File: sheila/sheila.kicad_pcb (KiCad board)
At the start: 2 copper layers, 53 parts, among them J1 PT_A, J10 GAIN1_RETURN, J11 OT1_A, J12 OT1_B, J13 SHIELD, J14 U1A_A_1, J15 U1A_K_3, J16 TS_T, J17 TS_B, J18 TS_M, J19 TS_GND, J2 PT_B, J20 U2_K_3, J21 GAIN1_GND, J22 U1A_G_2, J23 U2_S_9, J24 U2_A_7, J3 PT_CT, J4 S2_A, J5 S2_B, J7 U1B_6_A, J8 U1B_8_K, J9 GAIN1_SEND

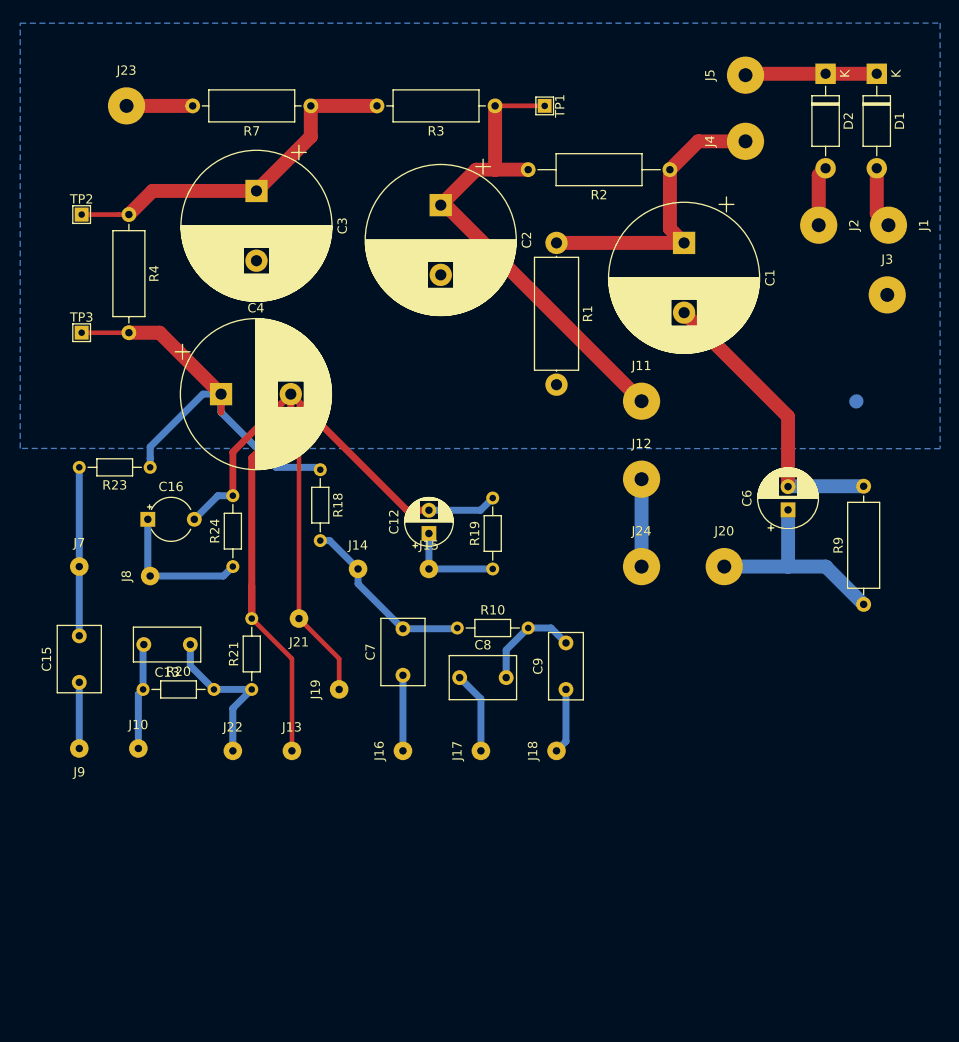
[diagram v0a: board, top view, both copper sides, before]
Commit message: .
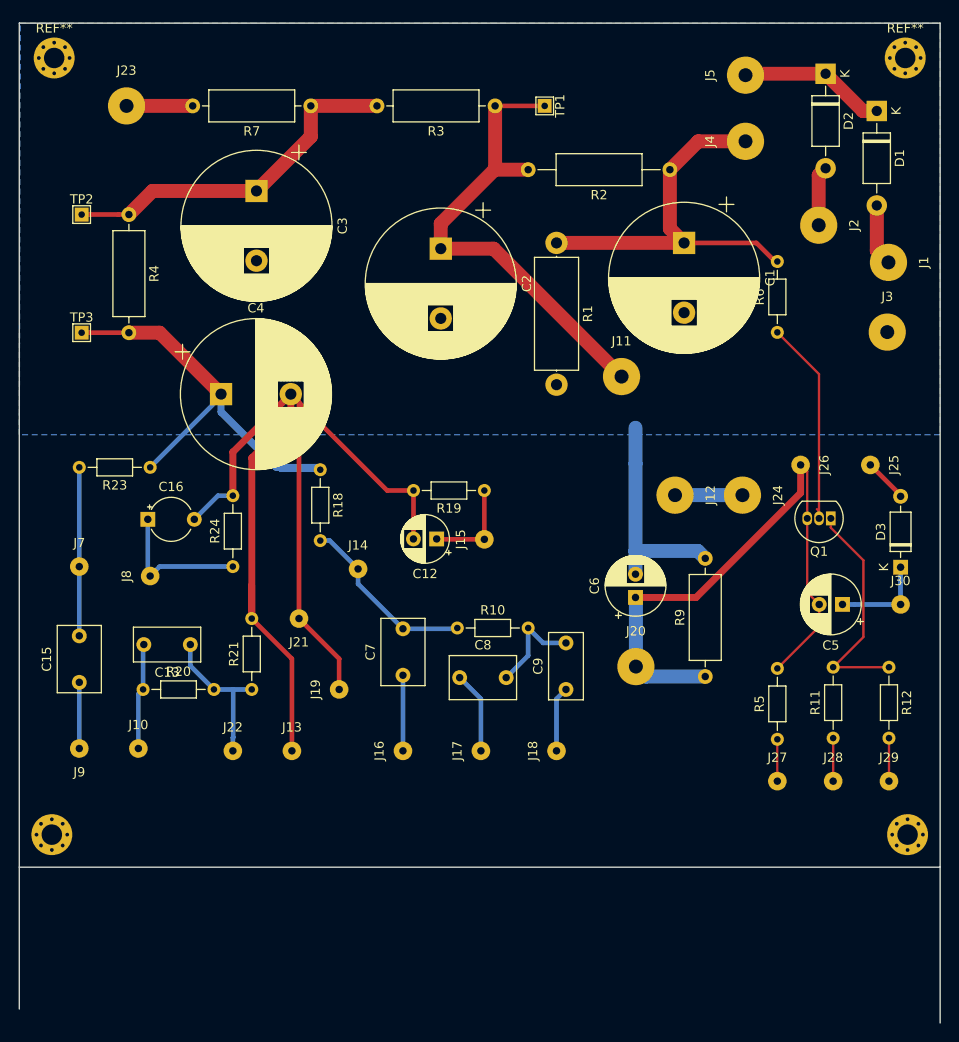
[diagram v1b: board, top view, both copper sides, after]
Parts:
- added C5: 220uF/16V, Capacitor_THT:CP_Radial_D6.3mm_P2.50mm, F.Cu at (190.0, 110.8)
- added D3: D_ALT, Diode_THT:D_DO-35_SOD27_P7.62mm_Horizontal, F.Cu at (196.2, 106.8)
- added J25: PT_H1, Connector_Wire:SolderWirePad_1x01_Drill0.8mm, F.Cu at (193.0, 95.8)
- added J26: PT_H2, Connector_Wire:SolderWirePad_1x01_Drill0.8mm, F.Cu at (185.5, 95.8)
- added J27: LED1_R, Connector_Wire:SolderWirePad_1x01_Drill0.8mm, F.Cu at (183.0, 129.8)
- added J28: LED1_G, Connector_Wire:SolderWirePad_1x01_Drill0.8mm, F.Cu at (189.0, 129.8)
- added J29: LED1_B, Connector_Wire:SolderWirePad_1x01_Drill0.8mm, F.Cu at (195.0, 129.8)
- added J30: LED1_A, Connector_Wire:SolderWirePad_1x01_Drill0.8mm, F.Cu at (196.2, 110.8)
- added Q1: BC549, Package_TO_SOT_THT:TO-92_Inline, F.Cu at (188.8, 101.5)
- added R11: 1.2K, Resistor_THT:R_Axial_DIN0204_L3.6mm_D1.6mm_P7.62mm_Horizontal, F.Cu at (189.0, 125.1)
- added R12: 1.2K, Resistor_THT:R_Axial_DIN0204_L3.6mm_D1.6mm_P7.62mm_Horizontal, F.Cu at (195.0, 117.5)
- added R5: 1.2K, Resistor_THT:R_Axial_DIN0204_L3.6mm_D1.6mm_P7.62mm_Horizontal, F.Cu at (183.0, 125.2)
- added R6: 1M, Resistor_THT:R_Axial_DIN0204_L3.6mm_D1.6mm_P7.62mm_Horizontal, F.Cu at (183.0, 81.5)
- added REF**: MountingHole_2.2mm_M2_Pad_Via, MountingHole:MountingHole_2.2mm_M2_Pad_Via, F.Cu at (105.2, 52.0)
- added REF**: MountingHole_2.2mm_M2_Pad_Via, MountingHole:MountingHole_2.2mm_M2_Pad_Via, F.Cu at (105.0, 135.5)
- added REF**: MountingHole_2.2mm_M2_Pad_Via, MountingHole:MountingHole_2.2mm_M2_Pad_Via, F.Cu at (197.0, 135.5)
- added REF**: MountingHole_2.2mm_M2_Pad_Via, MountingHole:MountingHole_2.2mm_M2_Pad_Via, F.Cu at (196.8, 52.0)
- moved C6 18.9 mm to (167.8, 110.0)
- moved R9 18.7 mm to (175.2, 118.5)
- moved J20 14.3 mm to (167.8, 117.4)
- moved J24 13.3 mm to (179.2, 99.0), turned to 270 degrees
- moved R19 8.48 mm to (151.5, 98.5), turned to 180 degrees
- moved J15 6.76 mm to (151.5, 103.8), turned to 90 degrees
- moved C2 4.68 mm to (146.8, 72.5)
- moved D1 4.00 mm to (193.7, 57.7)
- moved J1 4.00 mm to (194.9, 74.0)
- moved J3 4.00 mm to (194.8, 81.5)
- moved J12 3.99 mm to (172.0, 99.0), turned to 270 degrees
- moved J11 3.41 mm to (166.2, 86.2)
- moved C12 1.02 mm to (146.4, 103.7), turned to 180 degrees
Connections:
- net Net-(C1-Pad1) renamed /B+
- net Net-(C6-Pad1) renamed /A
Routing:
- net /A: track 22.8 -> 65.3 mm
- net Net-(Q1-Pad1): track 0.00 -> 24.8 mm
- net Net-(Q1-Pad2): track 0.00 -> 22.9 mm
- net GND: track 157.0 -> 144.3 mm
- net /B+3: track 46.7 -> 58.6 mm
- net /B+: track 31.6 -> 42.6 mm
- net Net-(C5-Pad1): track 0.00 -> 10.2 mm
- net Net-(D3-Pad2): track 0.00 -> 4.73 mm
- net Net-(D4-Pad4): track 0.00 -> 4.63 mm
- net Net-(D4-Pad3): track 0.00 -> 4.63 mm
- net Net-(D4-Pad2): track 0.00 -> 4.50 mm
- net Net-(J12-Pad1): track 9.40 -> 7.25 mm
- net /B+1: track 53.5 -> 51.8 mm
- net Net-(D1-Pad1): track 14.2 -> 15.8 mm
- net Net-(C13-Pad1): track 17.4 -> 16.6 mm
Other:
- board outline added: 99 x 107.5 mm
